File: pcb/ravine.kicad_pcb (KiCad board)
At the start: 2 copper layers, 102 x 101.7 mm, 39 parts

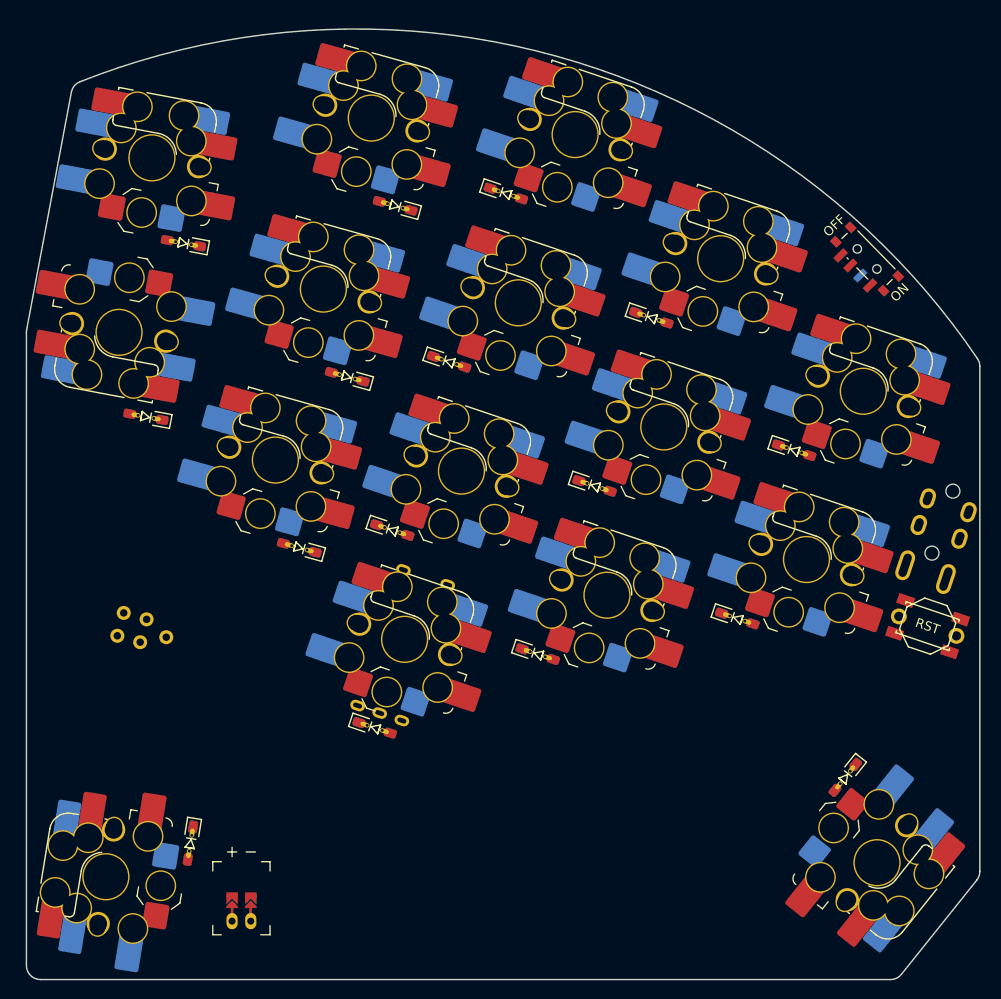
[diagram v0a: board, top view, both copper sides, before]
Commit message: okay last save before converting to normie matrix
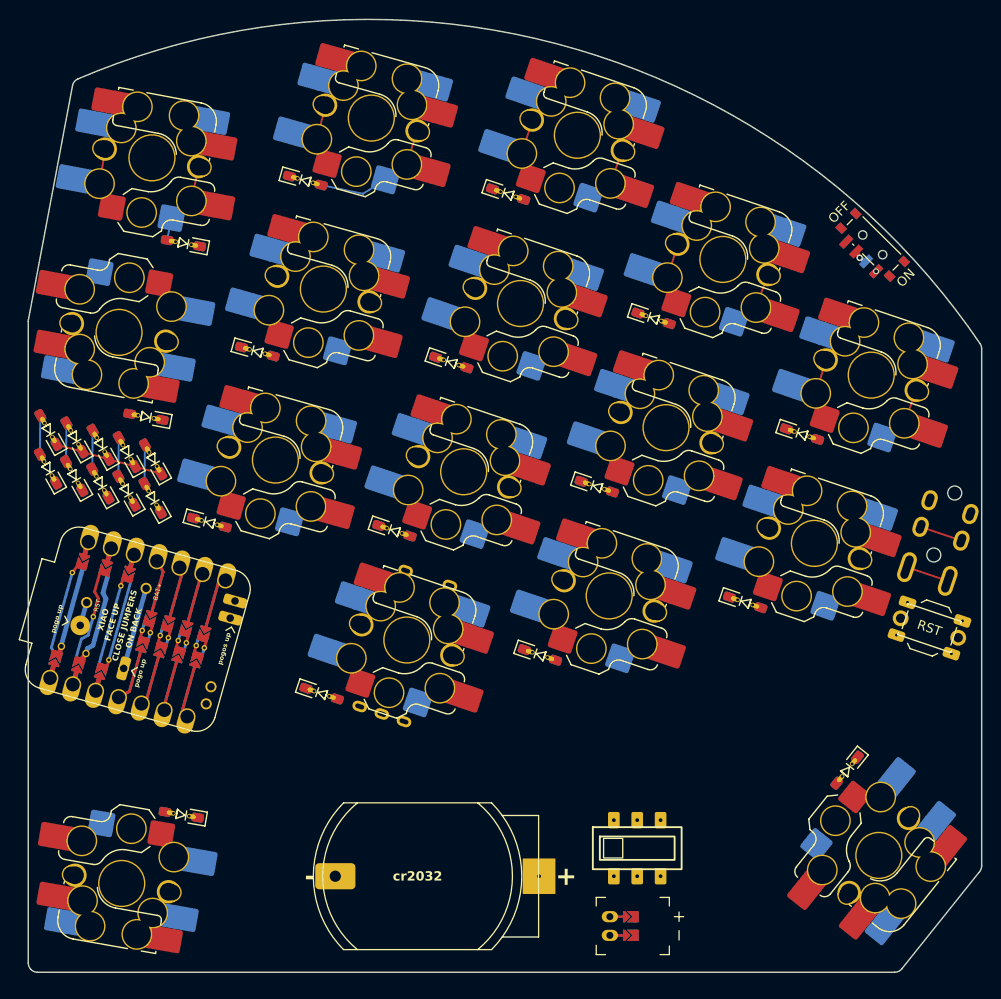
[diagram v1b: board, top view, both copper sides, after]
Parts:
- removed PLACEHOLDER: , placeholder
- added ?: , footprints:xiao-pogo-rev, F.Cu at (155.5, 163.1)
- added CR1: , footprints:bs-2032-8_rev, F.Cu at (185.5, 189.5)
- added D17: , footprints:diode_rev, F.Cu at (198.5, 165.8)
- added D18: , footprints:diode_rev, F.Cu at (204.6, 147.8)
- added D19: , footprints:diode_rev, F.Cu at (210.7, 129.8)
- added D20: , footprints:diode_rev, F.Cu at (220.5, 160.2)
- added D21: , footprints:diode_rev, F.Cu at (226.6, 142.2)
- added D22: , footprints:diode_rev, F.Cu at (231.4, 178.2)
- added D23: , footprints:diode_rev, F.Cu at (160.2, 182.9)
- added D24: , footprints:diode_rev, F.Cu at (160.4, 121.8)
- added D25: , footprints:diode_rev, F.Cu at (156.4, 140.4)
- added D26: , footprints:diode_rev, F.Cu at (175.2, 170.0)
- added XX1: , footprints:slider-mss22d18_rev, F.Cu at (209.0, 186.5)
- B1: footprint E73:SW_TACT_ALPS_SKQGABE010 -> footprints:alps-skqg_rev
- D1, D10, D11, D12, D13, D14, D15, D16, D2, D3, D4, D5, D6, D7, D8, D9: footprint diode-rev -> footprints:diode_rev
- SW1, SW10, SW11, SW12, SW13, SW14, SW15, SW16, SW2, SW3, SW4, SW5, SW6, SW7, SW8, SW9: footprint hs-mx-choc-rev -> footprints:hs-mx-choc_rev
- moved D9 79.9 mm to (157.1, 149.0), turned to 119.333 degrees
- moved D8 71.4 mm to (154.4, 144.1), turned to 119.333 degrees
- moved D7 66.8 mm to (154.3, 148.3), turned to 119.333 degrees
- moved D6 60.5 mm to (151.6, 143.3), turned to 119.333 degrees
- moved D16 58.8 mm to (195.1, 116.5), turned to -18.666 degrees
- moved D3 55.2 mm to (148.7, 146.7), turned to 119.333 degrees
- moved D4 54.7 mm to (148.8, 142.6), turned to 119.333 degrees
- moved D5 52.9 mm to (151.5, 147.5), turned to 119.333 degrees
- moved D2 43.5 mm to (146.0, 141.8), turned to 119.333 degrees
- moved D14 39.9 mm to (183.0, 152.6), turned to -18.6667 degrees
- moved JST1 39.4 mm to (206.0, 194.8), turned to 90 degrees
- moved D1 37.4 mm to (145.9, 145.9), turned to 119.333 degrees
- moved D15 33.2 mm to (189.1, 134.6), turned to -18.6667 degrees
- moved D10 23.4 mm to (157.2, 144.9), turned to 119.333 degrees
- moved D11 10.0 mm to (163.2, 151.7), turned to -15.6667 degrees
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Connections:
- D1 pad 1: middle_bottom -> D6
- D1 pad 2: (no net) -> P6
- D10 pad 1: pinky_top -> D10
- D10 pad 2: P0 -> intr
- D11 pad 2: (no net) -> D9
- D12 pad 2: (no net) -> D9
- D13 pad 2: (no net) -> D9
- D14 pad 1: default_default -> middle_bottom
- D14 pad 2: P3 -> D8
- D15 pad 1: pinky_home -> middle_home
- D15 pad 2: P0 -> D8
- D16 pad 1: default_default -> middle_top
- D16 pad 2: P2 -> D8
- D2 pad 1: middle_home -> D6
- D2 pad 2: (no net) -> intr
- D3 pad 1: middle_top -> D7
- D3 pad 2: (no net) -> P7
- D4 pad 1: index_bottom -> D7
- D4 pad 2: P3 -> intr
- D5 pad 1: index_home -> D8
- D5 pad 2: P3 -> P8
- D6 pad 1: index_top -> D8
- D6 pad 2: P3 -> intr
- D7 pad 1: inner_home -> D9
- D7 pad 2: P4 -> P9
- D8 pad 1: inner_top -> D9
- D8 pad 2: P4 -> intr
- D9 pad 1: default_default -> D10
- D9 pad 2: P0 -> P10
- JST1 pad 1: battery -> jst_bat
- RE1 pad S1: default_default -> P7
- RE1 pad S2: P3 -> default_default
- SW1 pad 1: P1 -> P9
- SW10 pad 1: P1 -> P9
- SW11 pad 1: P0 -> P10
- SW12 pad 1: P1 -> P9
- SW13 pad 1: P0 -> P10
- SW14 pad 1: P3 -> P7
- SW15 pad 1: P3 -> P7
- SW15 pad 2: default_default -> thumb_default
- SW16 pad 1: P4 -> P6
- SW2 pad 1: P0 -> P6
- SW3 pad 1: P2 -> P8
- SW4 pad 1: P4 -> P6
- SW5 pad 1: P0 -> P10
- SW6 pad 1: P4 -> P6
- SW7 pad 1: P1 -> P9
- SW8 pad 1: P0 -> P10
- SW9 pad 1: P2 -> P8
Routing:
- net P10: track 0.00 -> 15.0 mm
- net intr: track 0.00 -> 11.6 mm
- net ring_top: track 0.00 -> 11.1 mm
- net pinky_top: track 0.00 -> 6.15 mm
- net trrs: track 0.00 -> 4.60 mm
- net VCC: track 0.00 -> 4.60 mm
- net D7: track 0.00 -> 4.12 mm
- net D10: track 0.00 -> 4.12 mm
- net D8: track 0.00 -> 4.12 mm
- net D6: track 0.00 -> 4.12 mm
- net D9: track 0.00 -> 4.12 mm
- net middle_top: track 0.00 -> 3.75 mm
- net inner_top: track 0.00 -> 3.75 mm
- net index_top: track 0.00 -> 3.75 mm
- net P6: track 0.00 -> 3.75 mm
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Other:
- board size 102 x 101.7 mm -> 102 x 101.9 mm
